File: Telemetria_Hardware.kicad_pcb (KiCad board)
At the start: 2 copper layers, 27 parts, among them M100A1 1715734, SW1 RESET BUTTON, U1 CA3140, U2 CA3140

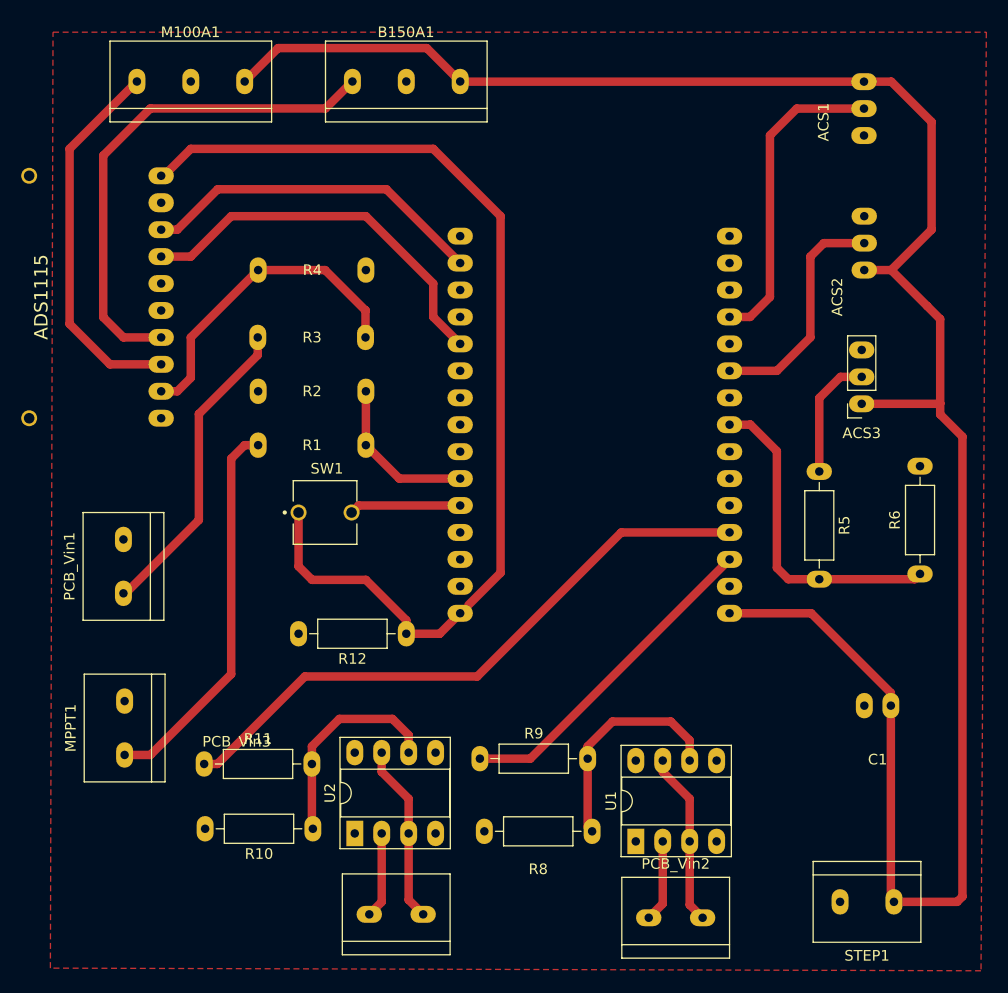
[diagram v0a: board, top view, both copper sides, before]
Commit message: sugestao
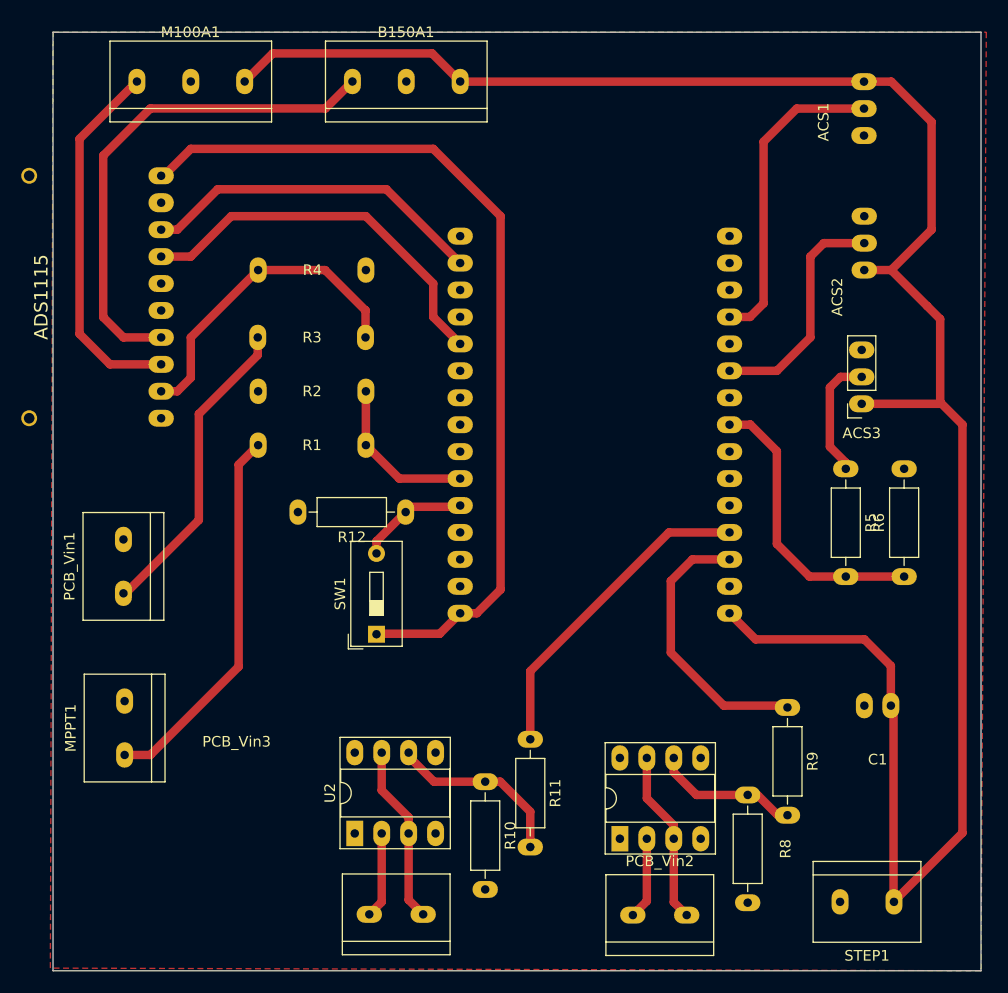
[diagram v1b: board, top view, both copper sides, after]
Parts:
- SW1: value RESET BUTTON -> SW_SPST; footprint BUTT:BUTT -> Button_Switch_THT:SW_DIP_SPSTx01_Slide_9.78x4.72mm_W7.62mm_P2.54mm
- moved R11 30.8 mm to (110.8, 119.2), turned to -90 degrees
- moved R9 29.4 mm to (135.0, 116.2), turned to -90 degrees
- moved R10 16.8 mm to (106.5, 123.2), turned to -90 degrees
- moved R8 15.1 mm to (131.2, 124.4), turned to -90 degrees
- moved SW1 12.5 mm to (96.2, 109.3), turned to 90 degrees
- moved R12 11.5 mm to (99.0, 97.8)
- moved R5 2.51 mm to (140.5, 93.7)
- moved PCB_Vin2 1.52 mm to (120.4, 135.8)
- moved R6 1.52 mm to (146.0, 103.8)
- moved U1 1.52 mm to (119.2, 128.6)
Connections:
- ESP32 pad 20: Net-(ADS1115-VDD) -> Net-(ESP32-IO4)
- R12 pad 1: Net-(ADS1115-VDD) -> Net-(ESP32-IO4)
- SW1 pad 2: Net-(ADS1115-VDD) -> Net-(ESP32-IO4)
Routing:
- net Net-(ESP32-IO12): track 58.6 -> 30.6 mm
- net Net-(ADS1115-VDD): track 108.6 -> 84.3 mm
- net Net-(ESP32-IO4): track 0.00 -> 10.4 mm
- net Net-(R8-Pad1): track 21.5 -> 13.7 mm
- net Net-(ESP32-IO13): track 31.3 -> 26.3 mm
- net Net-(R10-Pad1): track 20.3 -> 17.3 mm
- net Net-(ESP32-IO25): track 30.2 -> 27.5 mm
- net Net-(ACS1-Pin_1): track 201.1 -> 198.8 mm
- net Net-(ADS1115-A1): track 35.7 -> 34.9 mm
- net Net-(MPPT1-Pad1): track 36.6 -> 35.8 mm
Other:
- board outline added: 87.5 x 88.5 mm
